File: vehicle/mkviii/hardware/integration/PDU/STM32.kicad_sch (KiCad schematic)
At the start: 68 parts, among them J7 CONN_02X03, U1 STM32G441CBTx, U2 MCP23S17_SS, U20 ADC1283, U21 MAX7221xNG, U4 CC56-12SEKWA, U6 MCP2561-E_SN, Y1 Crystal_SMD

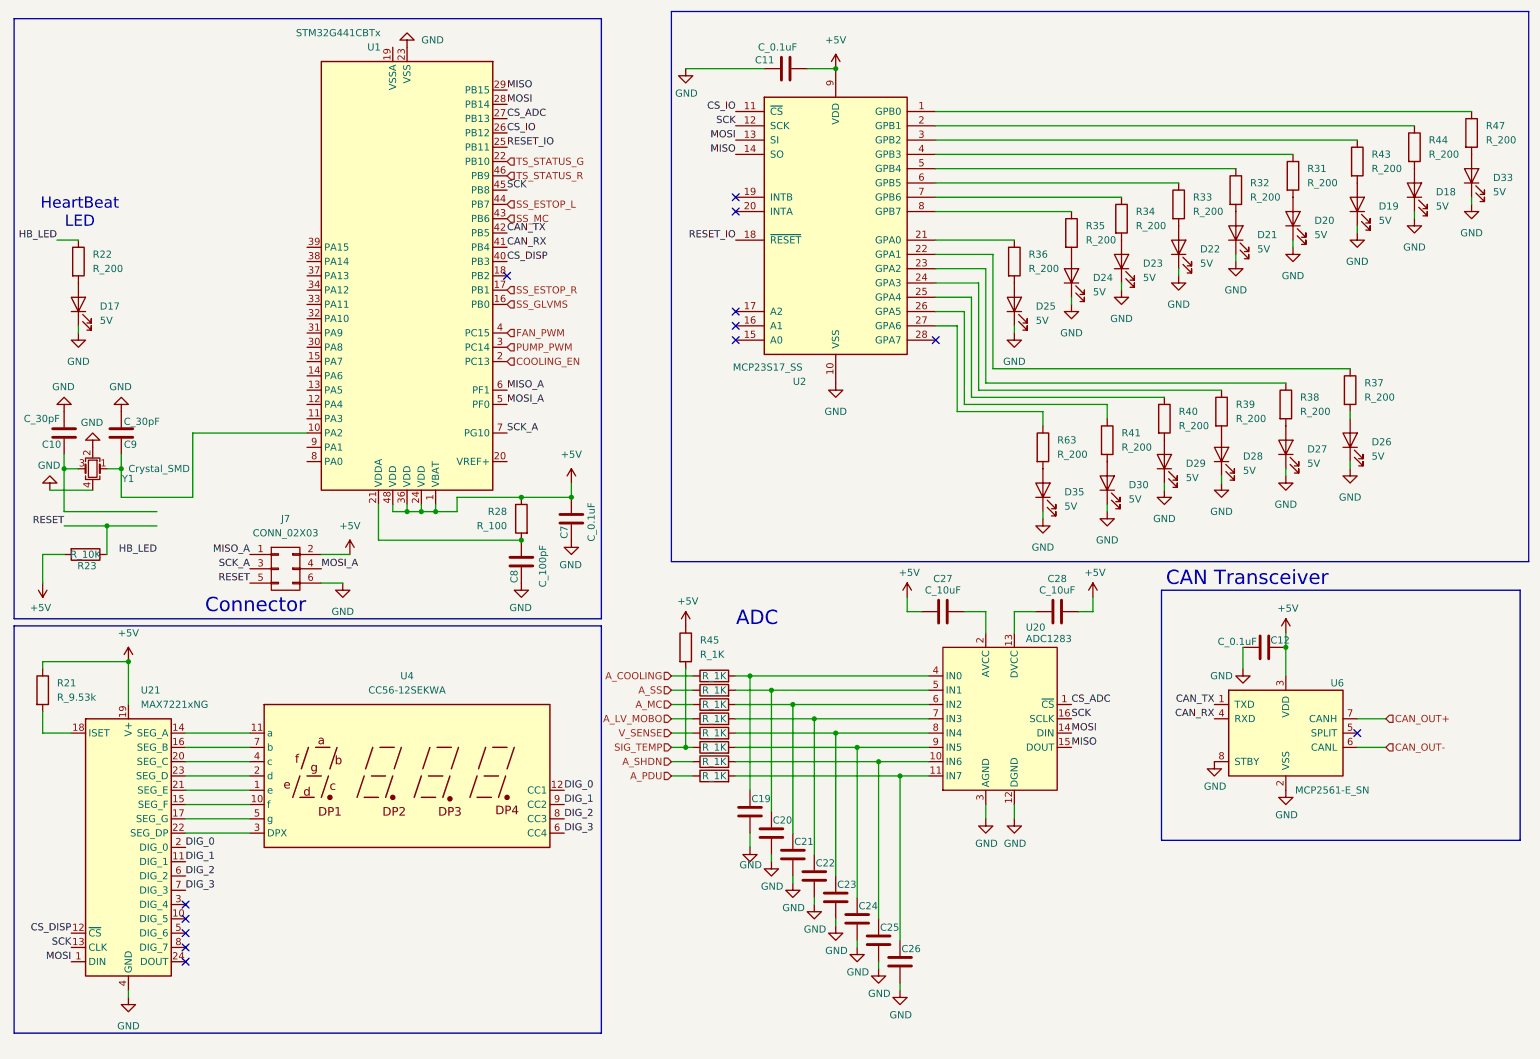
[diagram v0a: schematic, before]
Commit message: Fix the STM32 schematic
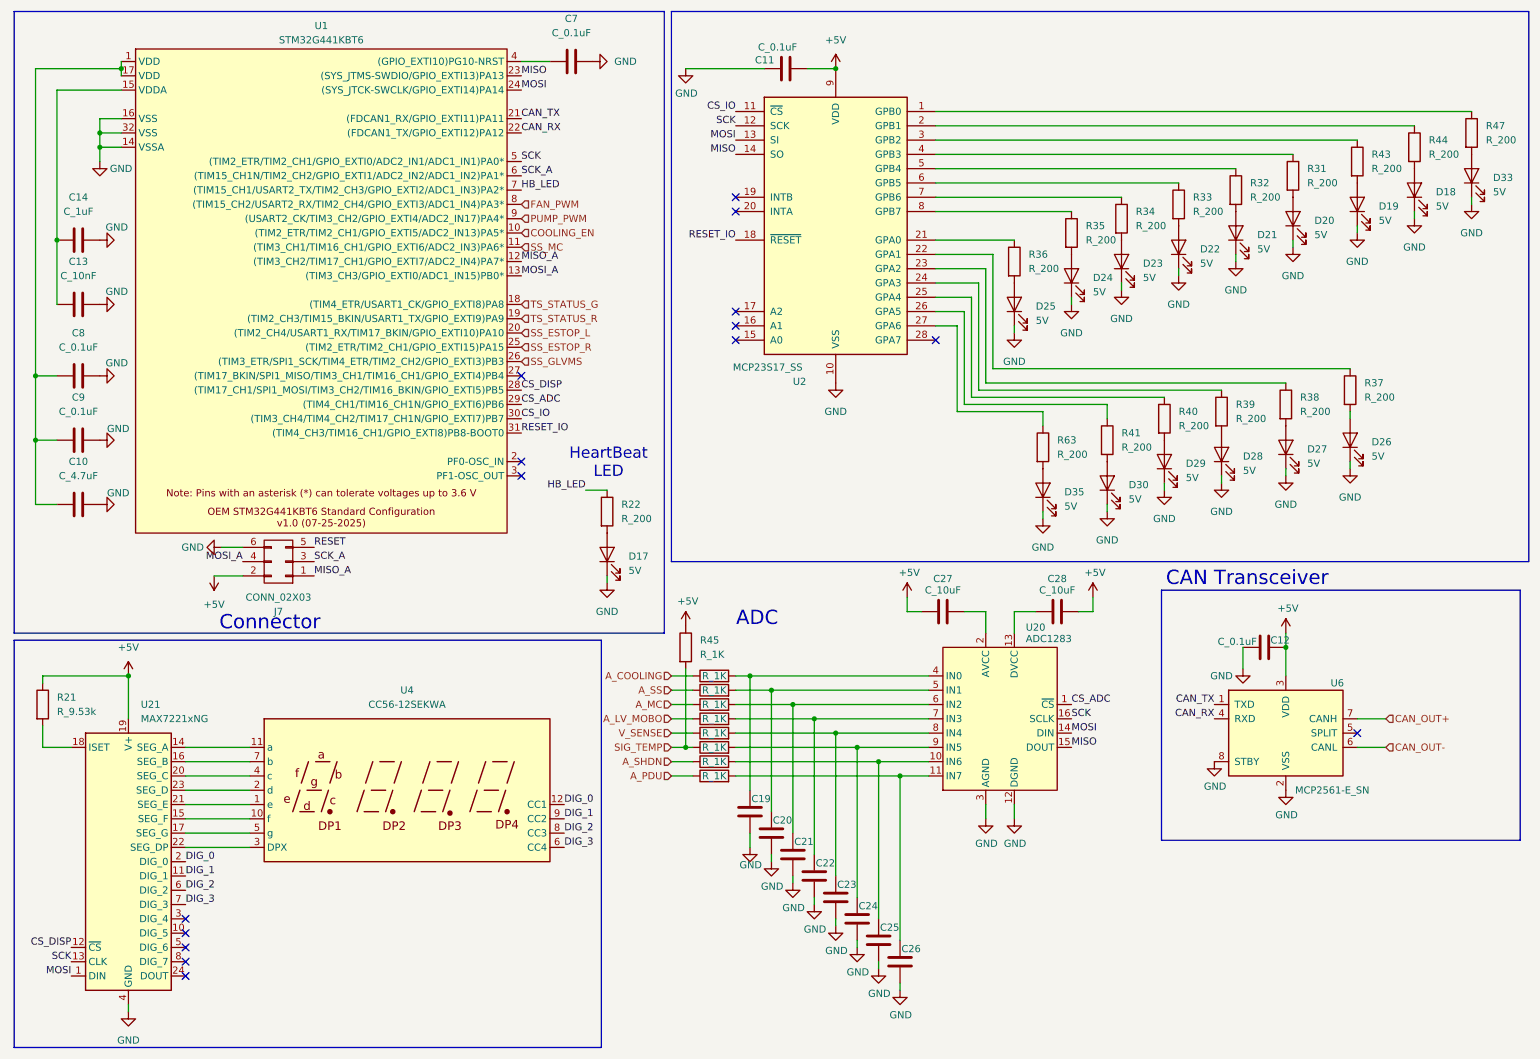
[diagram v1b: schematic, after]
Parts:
- removed C10, C9: C_30pF, OEM:C_0603_1608Metric, symbol formula:C_30pF
- removed C7: C_0.1uF, OEM:C_0603_1608Metric, symbol formula:C_0.1uF
- removed C8: C_100pF, OEM:C_0603_1608Metric, symbol formula:C_100pF
- removed R23: R_10K, OEM:R_0603, symbol OEM:R_10K
- removed R28: R_100, OEM:R_0603, symbol OEM:R_100
- removed U1: STM32G441CBTx, Package_QFP:LQFP-48_7x7mm_P0.5mm, symbol MCU_ST_STM32G4:STM32G441CBTx
- removed Y1: Crystal_SMD, OEM:Crystal_SMD_FA238, symbol formula:Crystal_SMD
- added C10: C_4.7uF, Capacitor_SMD:C_0603_1608Metric, symbol OEM:C_4.7uF_20-100V_0603
- added C13: C_10nF, Capacitor_SMD:C_0603_1608Metric, symbol OEM:C_10nF_20-100V_0603
- added C14: C_1uF, Capacitor_SMD:C_0603_1608Metric, symbol OEM:C_1uF_20-100V_0603
- added C7, C8, C9: C_0.1uF, Capacitor_SMD:C_0603_1608Metric, symbol OEM:C_0.1uF_0-20V_0603
- added U1: STM32G441KBT6, Package_QFP:LQFP-32_7x7mm_P0.8mm, symbol OEM:U_MCU_STM32G441KBT6_32-LQFP
- D17: footprint OEM:CHIPLED_0805 -> LED_SMD:LED_0805_2012Metric
- R22: footprint OEM:R_0603 -> Resistor_SMD:R_0603_1608Metric
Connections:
- net CAN_RX: now also U1.22 ((FDCAN1_TX/GPIO_EXTI12)PA12)
- net CAN_TX: now also U1.21 ((FDCAN1_RX/GPIO_EXTI11)PA11)
- net COOLING_EN: now also U1.10 ((TIM2_ETR/TIM2_CH1/GPIO_EXTI5/ADC2_IN13)PA5*)
- net CS_ADC: now also U1.29 ((TIM4_CH1/TIM16_CH1N/GPIO_EXTI6)PB6)
- net CS_DISP: now also U1.28 ((TIM17_CH1/SPI1_MOSI/TIM3_CH2/TIM16_BKIN/GPIO_EXTI5)PB5)
- net CS_IO: now also U1.30 ((TIM3_CH4/TIM4_CH2/TIM17_CH1N/GPIO_EXTI7)PB7)
- net FAN_PWM: now also U1.8 ((TIM15_CH2/USART2_RX/TIM2_CH4/GPIO_EXTI3/ADC1_IN4)PA3*)
- net GND: now also C10.2, C13.2, C14.2, C7.2, C8.2, C9.2, U1.14 (VSSA), U1.16 (VSS), U1.32 (VSS)
- net HB_LED: now also U1.7 ((TIM15_CH1/USART2_TX/TIM2_CH3/GPIO_EXTI2/ADC1_IN3)PA2*)
- net MISO: now also U1.23 ((SYS_JTMS-SWDIO/GPIO_EXTI13)PA13)
- net MISO_A: now also U1.12 ((TIM3_CH2/TIM17_CH1/GPIO_EXTI7/ADC2_IN4)PA7*)
- net MOSI: now also U1.24 ((SYS_JTCK-SWCLK/GPIO_EXTI14)PA14)
- net MOSI_A: now also U1.13 ((TIM3_CH3/GPIO_EXTI0/ADC1_IN15)PB0*)
- net PUMP_PWM: now also U1.9 ((USART2_CK/TIM3_CH2/GPIO_EXTI4/ADC2_IN17)PA4*)
- net RESET_IO: now also U1.31 ((TIM4_CH3/TIM16_CH1/GPIO_EXTI8)PB8-BOOT0)
- net SCK: now also U1.5 ((TIM2_ETR/TIM2_CH1/GPIO_EXTI0/ADC2_IN1/ADC1_IN1)PA0*)
- net SCK_A: now also U1.6 ((TIM15_CH1N/TIM2_CH2/GPIO_EXTI1/ADC2_IN2/ADC1_IN2)PA1*)
- net SS_ESTOP_L: now also U1.20 ((TIM2_CH4/USART1_RX/TIM17_BKIN/GPIO_EXTI10)PA10)
- net SS_ESTOP_R: now also U1.25 ((TIM2_ETR/TIM2_CH1/GPIO_EXTI15)PA15)
- net SS_GLVMS: now also U1.26 ((TIM3_ETR/SPI1_SCK/TIM4_ETR/TIM2_CH2/GPIO_EXTI3)PB3)
- net SS_MC: now also U1.11 ((TIM3_CH1/TIM16_CH1/GPIO_EXTI6/ADC2_IN3)PA6*)
- net TS_STATUS_G: now also U1.18 ((TIM4_ETR/USART1_CK/GPIO_EXTI8)PA8)
- net TS_STATUS_R: now also U1.19 ((TIM2_CH3/TIM15_BKIN/USART1_TX/GPIO_EXTI9)PA9)
- new net: C10.1, C8.1, C9.1, U1.1 (VDD), U1.17 (VDD)
- new net: C13.1, C14.1, U1.15 (VDDA)
- new net: C7.1, U1.4 ((GPIO_EXTI10)PG10-NRST)
- no-connect marks 13 -> 15
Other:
- moved on the sheet: D17, J7, R21, R22, U21, U4
